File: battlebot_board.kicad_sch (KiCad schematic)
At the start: 42 parts, among them J1 Conn_01x02_Pin, J2 Conn_01x04_Pin, J3 JST_SMD_1.0mm_Vertical, J4 Conn_01x02, J5 JST_02, J6 JST_02, Q1 AO3400A, Q2 AO3400A, SW1 Switch_Tactile_CnK, U1 AP63203WU, U2 LPC824M201JHI33, U3 TMP102, U4 LSM6DSOX, U5 W25Q128JVP

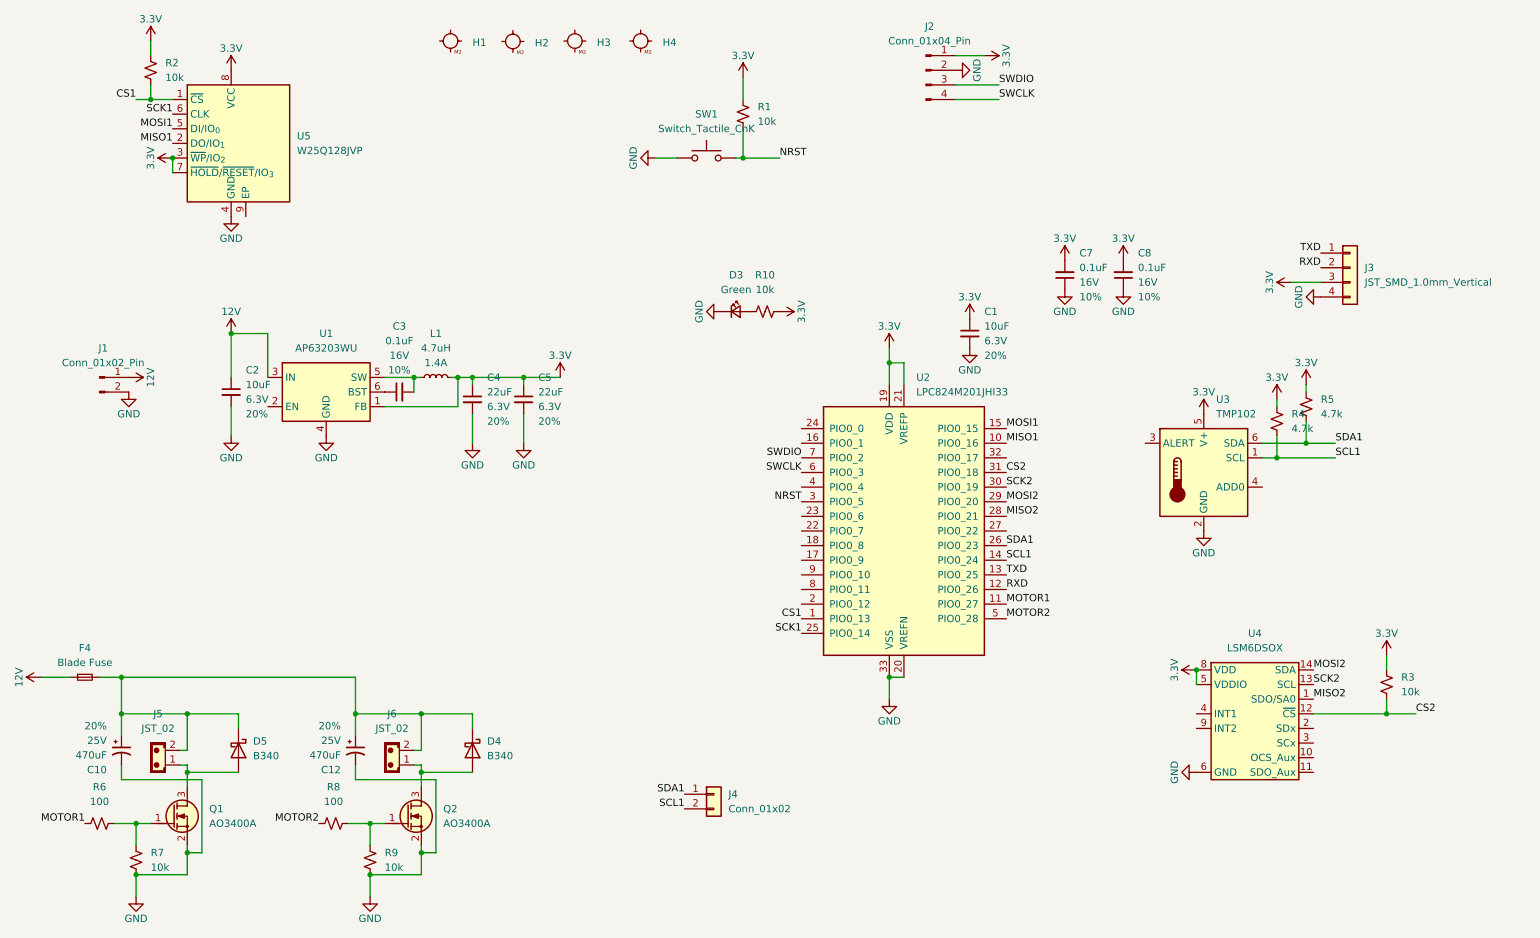
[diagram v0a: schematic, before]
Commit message: redesign
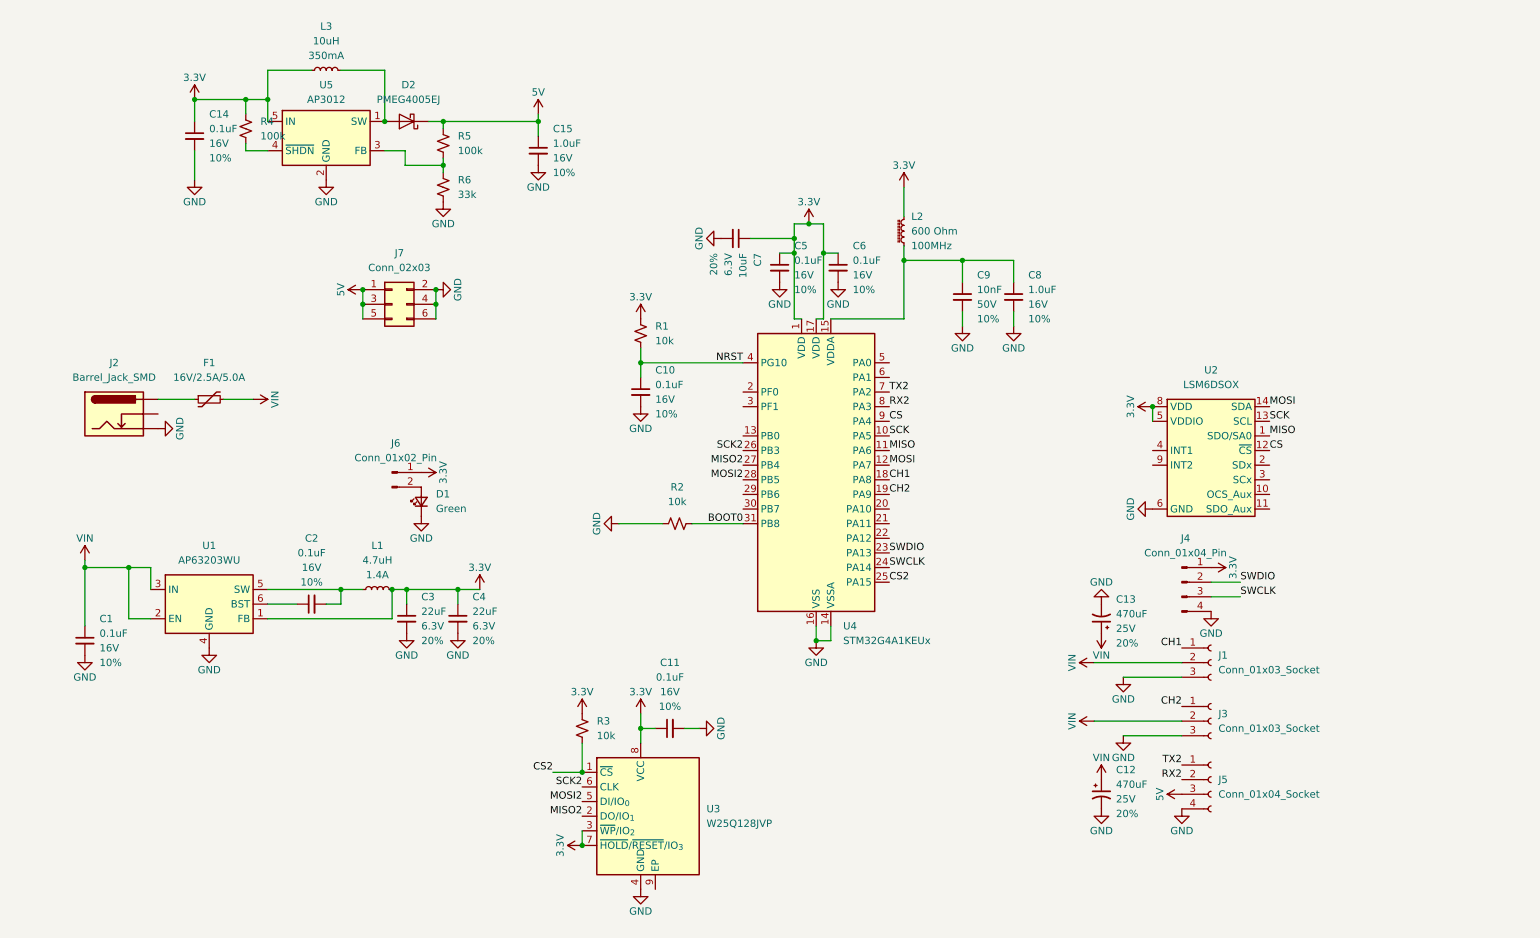
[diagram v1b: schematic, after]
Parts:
- removed C1, C2: 10uF, PCM_SparkFun-Capacitor:C_0402_1005Metric, symbol PCM_SparkFun-Capacitor:10uF_0402_6.3V_20%
- removed C10: 470uF, PCM_SparkFun-Capacitor:Electrolytic_10.3x10.3mm, symbol PCM_SparkFun-Capacitor:470uF_10x10_25V_20%
- removed C3, C7, C8: 0.1uF, PCM_SparkFun-Capacitor:C_0402_1005Metric, symbol PCM_SparkFun-Capacitor:0.1uF_0402_16V_10%
- removed C5: 22uF, PCM_SparkFun-Capacitor:C_0603_1608Metric, symbol PCM_SparkFun-Capacitor:22uF_0603_6.3V_20%
- removed D3: Green, PCM_SparkFun-LED:LED_0603_1608Metric_Green, symbol PCM_SparkFun-LED:LED_Green_0603
- removed D4, D5: B340, Diode_SMD:D_SMC, symbol Diode:B340
- removed F4: Blade Fuse, PCM_SparkFun-Fuse:Fuseholder_Automotive, symbol PCM_SparkFun-Fuse:Fuse_Holder-Blade
- removed H1, H2, H3, H4: (no value), PCM_fab:MountingHole_M2, symbol PCM_fab:MountingHole_M2
- removed J1: Conn_01x02_Pin, Connector_JST:JST_EH_B2B-EH-A_1x02_P2.50mm_Vertical, symbol Connector:Conn_01x02_Pin
- removed J2: Conn_01x04_Pin, Connector_JST:JST_EH_B4B-EH-A_1x04_P2.50mm_Vertical, symbol Connector:Conn_01x04_Pin
- removed J3: JST_SMD_1.0mm_Vertical, PCM_SparkFun-Connector:JST_1x04_P1.0mm_Vertical_SMD, symbol PCM_SparkFun-Connector:Conn_01x04_JST_P1.0mm_Vertical_SMD
- removed J4: Conn_01x02, Connector_JST:JST_EH_B2B-EH-A_1x02_P2.50mm_Vertical, symbol PCM_4ms_Connector:Conn_01x02
- removed J5, J6: JST_02, Connector_JST:JST_EH_B2B-EH-A_1x02_P2.50mm_Vertical, symbol PCM_SL_Connectors:JST_02
- removed Q1, Q2: AO3400A, Package_TO_SOT_SMD:SOT-23, symbol PCM_Transistor_MOSFET_AKL:AO3400A
- removed R10, R7, R9: 10k, PCM_SparkFun-Resistor:R_0402_1005Metric, symbol PCM_SparkFun-Resistor:10k_0402
- removed R4, R5: 4.7k, PCM_SparkFun-Resistor:R_0402_1005Metric, symbol PCM_SparkFun-Resistor:4.7k_0402
- removed R6, R8: 100, PCM_SparkFun-Resistor:R_0402_1005Metric, symbol PCM_SparkFun-Resistor:100_0402
- removed SW1: Switch_Tactile_CnK, PCM_fab:Button_CnK_PTS636.0_6x3.5mm, symbol PCM_fab:Switch_Tactile_CnK
- removed U2: LPC824M201JHI33, Package_DFN_QFN:QFN-32-1EP_5x5mm_P0.5mm_EP3.45x3.45mm, symbol MCU_NXP_LPC:LPC824M201JHI33
- removed U3: TMP102, PCM_SparkFun-Semiconductor-Standard:SOT-563, symbol PCM_SparkFun-Sensor:TMP102
- removed U4: LSM6DSOX, PCM_SparkFun-Sensor:ST_LGA-14L_2.5x3.0mm_P0.5mm_4x3, symbol PCM_SparkFun-Sensor:LSM6DSOX
- removed U5: W25Q128JVP, Package_SON:WSON-8-1EP_6x5mm_P1.27mm_EP3.4x4.3mm, symbol Memory_Flash:W25Q128JVP
- added C1, C10, C11, C14, C2, C5, C6: 0.1uF, PCM_SparkFun-Capacitor:C_0402_1005Metric, symbol PCM_SparkFun-Capacitor:0.1uF_0402_16V_10%
- added C13: 470uF, PCM_SparkFun-Capacitor:Electrolytic_10.3x10.3mm, symbol PCM_SparkFun-Capacitor:470uF_10x10_25V_20%
- added C15, C8: 1.0uF, PCM_SparkFun-Capacitor:C_0402_1005Metric, symbol PCM_SparkFun-Capacitor:1.0uF_0402_16V_10%
- added C3: 22uF, PCM_SparkFun-Capacitor:C_0603_1608Metric, symbol PCM_SparkFun-Capacitor:22uF_0603_6.3V_20%
- added C7: 10uF, PCM_SparkFun-Capacitor:C_0402_1005Metric, symbol PCM_SparkFun-Capacitor:10uF_0402_6.3V_20%
- added C9: 10nF, PCM_SparkFun-Capacitor:C_0402_1005Metric, symbol PCM_SparkFun-Capacitor:10nF_0402_25V_10%
- added D1: Green, PCM_SparkFun-LED:LED_0603_1608Metric_Green, symbol PCM_SparkFun-LED:LED_Green_0603
- added D2: PMEG4005EJ, Diode_SMD:D_SOD-323F, symbol Diode:PMEG4005EJ
- added F1: 16V/2.5A/5.0A, PCM_SparkFun-Fuse:1812, symbol PCM_SparkFun-Fuse:Fuse 16V/2.5A/5.0A
- added J1, J3: Conn_01x03_Socket, PCM_SparkFun-Connector:JST_1x03_P1.0mm_Vertical_SMD, symbol Connector:Conn_01x03_Socket
- added J2: Barrel_Jack_SMD, PCM_SparkFun-Connector:Barrel_Jack_SMD, symbol PCM_SparkFun-Connector:Barrel_Jack_SMD
- added J4: Conn_01x04_Pin, Connector_PinHeader_1.27mm:PinHeader_1x04_P1.27mm_Vertical, symbol Connector:Conn_01x04_Pin
- added J5: Conn_01x04_Socket, PCM_SparkFun-Connector:JST_1x04_P1.0mm_Vertical_SMD, symbol Connector:Conn_01x04_Socket
- added J6: Conn_01x02_Pin, Connector_PinHeader_1.27mm:PinHeader_1x02_P1.27mm_Vertical, symbol Connector:Conn_01x02_Pin
- added J7: Conn_02x03, Connector_PinHeader_1.27mm:PinHeader_2x03_P1.27mm_Vertical, symbol PCM_4ms_Connector:Conn_02x03
- added L2: 600 Ohm, PCM_SparkFun-Capacitor:C_0805_2012Metric, symbol PCM_SparkFun-Coil:Ferrite_600Ohm_0805_500mA
- added L3: 10uH, PCM_SparkFun-Capacitor:C_0805_2012Metric, symbol PCM_SparkFun-Coil:10uH_0805_0.35A
- added R4, R5: 100k, PCM_SparkFun-Resistor:R_0402_1005Metric, symbol PCM_SparkFun-Resistor:100k_0402
- added R6: 33k, PCM_SparkFun-Resistor:R_0402_1005Metric, symbol PCM_SparkFun-Resistor:33k_0402
- added U2: LSM6DSOX, PCM_SparkFun-Sensor:ST_LGA-14L_2.5x3.0mm_P0.5mm_4x3, symbol PCM_SparkFun-Sensor:LSM6DSOX
- added U3: W25Q128JVP, Package_SON:WSON-8-1EP_6x5mm_P1.27mm_EP3.4x4.3mm, symbol Memory_Flash:W25Q128JVP
- added U4: STM32G4A1KEUx, Package_DFN_QFN:QFN-32-1EP_5x5mm_P0.5mm_EP3.45x3.45mm, symbol MCU_ST_STM32G4:STM32G4A1KEUx
- added U5: AP3012, PCM_SparkFun-Semiconductor-Standard:SOT23-5, symbol PCM_SparkFun-IC-Power:AP3012
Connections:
- net 12V is gone; now on net VIN: U1.3 (IN)
- net CS1 is gone; now on net GND: R2.1
- net 3.3V: now also C11.1, C14.1, C3.1, C5.1, C6.1, C7.1, J4.1 (Pin_1), J6.1 (Pin_1), L2.2, L3.1, R4.2, U2.5 (VDDIO), U2.8 (VDD), U3.3 (~{WP}/IO_{2}), U3.7 (~{HOLD}/~{RESET}/IO_{3}), U3.8 (VCC), U4.1 (VDD), U4.17 (VDD), U5.5 (IN); no longer R2.2
- net CS2: now also U3.1 (~{CS}), U4.25 (PA15)
- net GND: now also C1.2, C10.2, C11.2, C13.2, C14.2, C15.2, C3.2, C5.2, C6.2, C7.2, C8.2, C9.2, D1.1 (K), J1.3 (Pin_3), J2.GND, J3.3 (Pin_3), J4.4 (Pin_4), J5.4 (Pin_4), J7.2 (+12V), J7.4 (GND), J7.6 (GND), R6.1, U2.6 (GND), U2.7 (GND), U3.4 (GND), U4.14 (VSSA), U4.16 (VSS), U4.32 (VSS), U4.33 (VSS), U5.2 (GND)
- net MISO2: now also U3.2 (DO/IO_{1}), U4.27 (PB4)
- net MOSI2: now also U3.5 (DI/IO_{0}), U4.28 (PB5)
- net NRST: now also C10.1, U4.4 (PG10)
- net SCK2: now also U3.6 (CLK), U4.26 (PB3)
- net SWCLK: now also J4.3 (Pin_3), U4.24 (PA14)
- net SWDIO: now also J4.2 (Pin_2), U4.23 (PA13)
- net VIN: now reaches C12.1
- net VIN: now also U1.2 (EN), C1.1, C13.1, F1.2, J1.2 (Pin_2), J3.2 (Pin_2)
- net at L1.1, U1.5 (SW): now also C2.2
- net at U1.6 (BST): now also C2.1
- new net: R4.1, U5.4 (~{SHDN})
- new net: C8.1, C9.1, L2.1, U4.15 (VDDA)
- new net: F1.1, J2.PWR
- new net: R5.1, R6.2, U5.3 (FB)
- new net: D1.2 (A), J6.2 (Pin_2)
- new net: D2.2 (A), L3.2, U5.1 (SW)
- new net 5V: C15.1, D2.1 (K), J5.3 (Pin_3), J7.1 (+12V), J7.3 (GND), J7.5 (GND), R5.2
- new net BOOT0: R2.2, U4.31 (PB8)
- new net CH1: J1.1 (Pin_1), U4.18 (PA8)
- new net CH2: J3.1 (Pin_1), U4.19 (PA9)
- new net CS: U2.12 (~{CS}), U4.9 (PA4)
- new net MISO: U2.1 (SDO/SA0), U4.11 (PA6)
- new net MOSI: U2.14 (SDA), U4.12 (PA7)
- new net RX2: J5.2 (Pin_2), U4.8 (PA3)
- new net SCK: U2.13 (SCL), U4.10 (PA5)
- new net TX2: J5.1 (Pin_1), U4.7 (PA2)
